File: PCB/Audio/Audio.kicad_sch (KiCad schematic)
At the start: 30 parts, among them J3 TC2030-USB-NL-DS, J4 TF_PUSH, J5 USB-C-Socket-H, U1 L, U2 ESP32-S3-MINI-1, U2 R, U5 MD8942

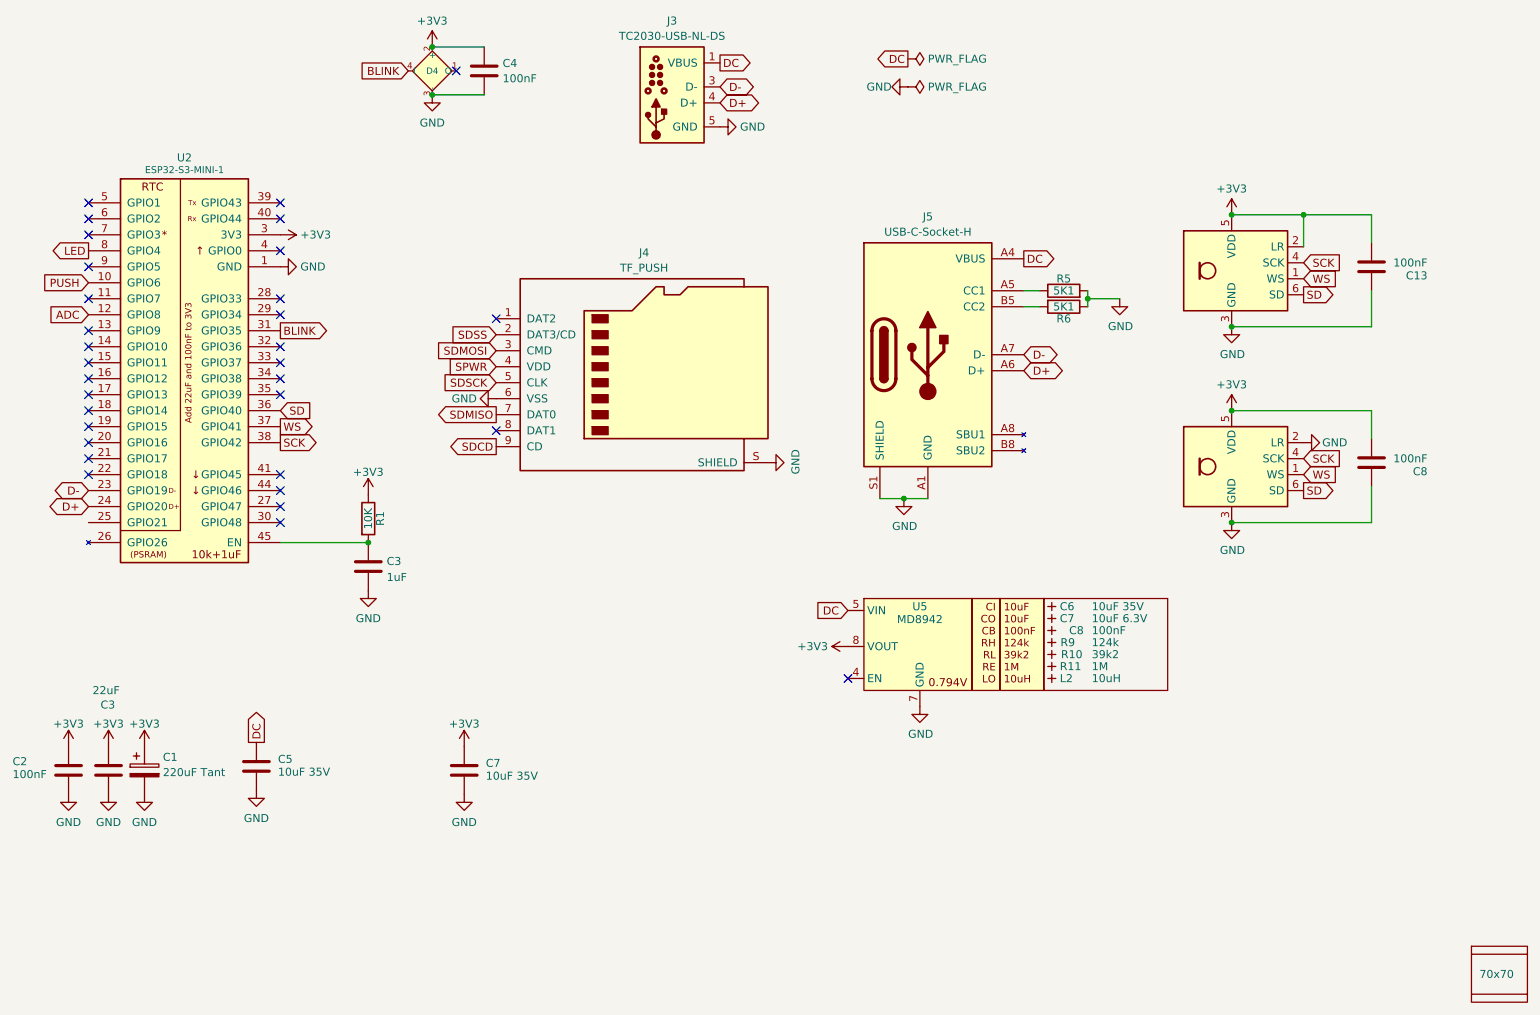
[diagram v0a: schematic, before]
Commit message: Rework concept
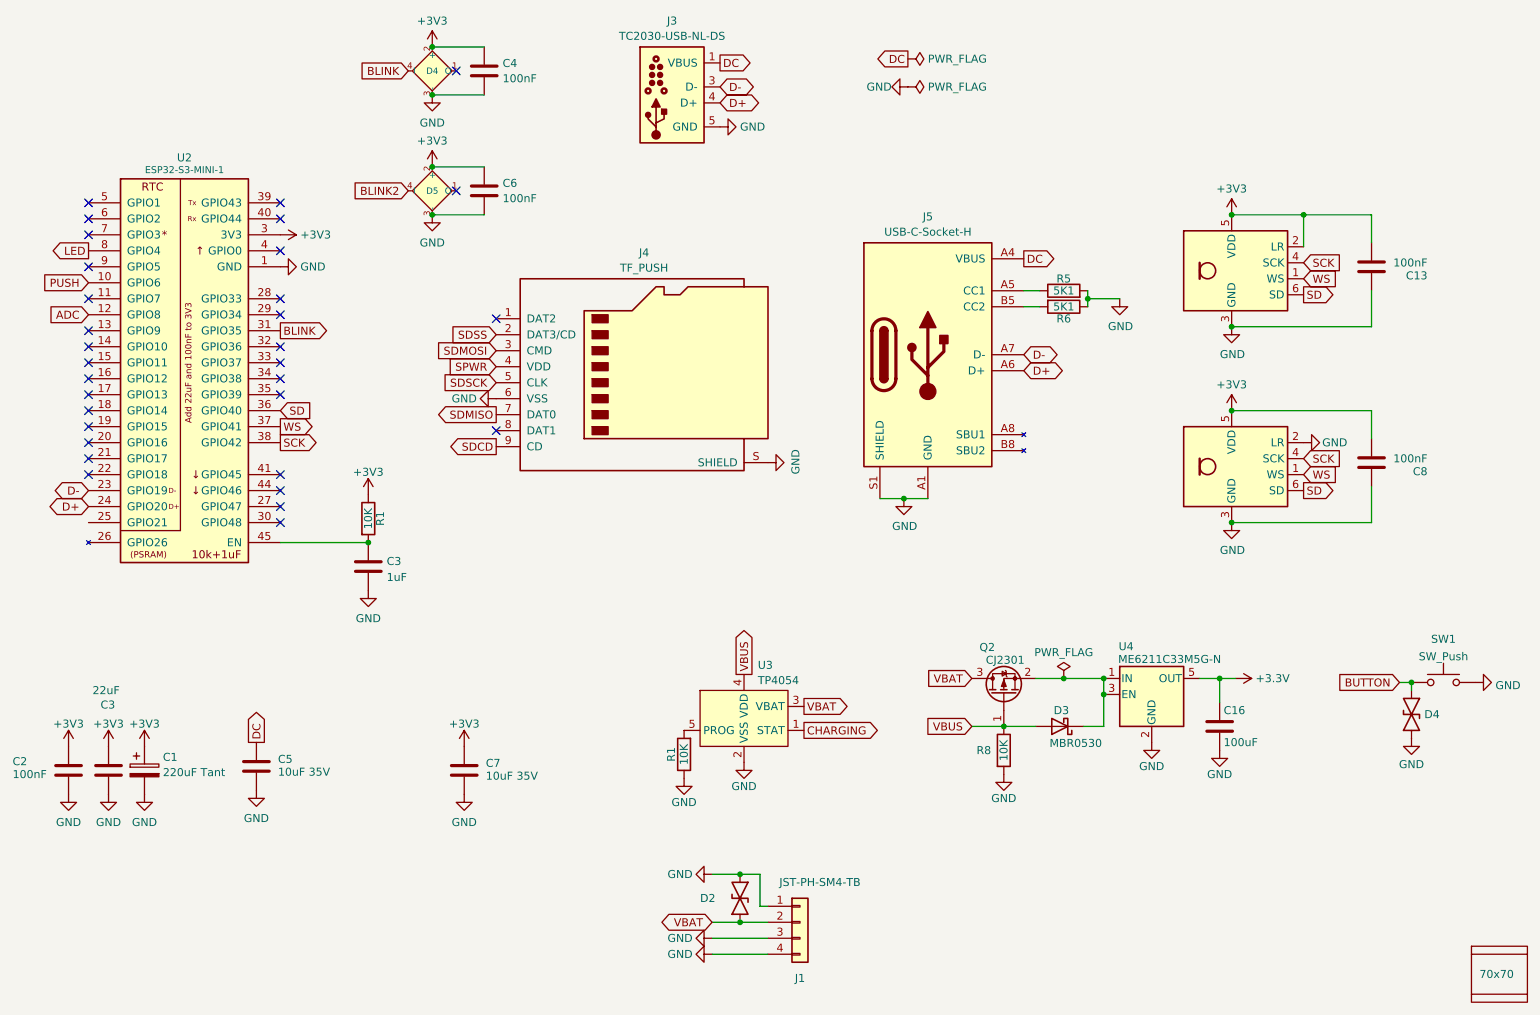
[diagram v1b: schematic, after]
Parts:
- removed C6: 10uF 35V, RevK:C_0603_, symbol RevK:Hidden
- removed C7: 10uF 6.3V, RevK:C_0603_, symbol RevK:Hidden
- removed C8: 100nF, RevK:C_0603_, symbol RevK:Hidden
- removed L2: 10uH, RevK:L_4x4_, symbol RevK:Hidden
- removed R10: 39k2, RevK:R_0402_, symbol RevK:Hidden
- removed R11: 1M, RevK:R_0402_, symbol RevK:Hidden
- removed R9: 124k, RevK:R_0402_, symbol RevK:Hidden
- removed U5: MD8942, RevK:SOT-23-6-MD8942, symbol RevK:MD89420-RegBlock
- added C16: 100uF, RevK:C_0805, symbol Device:C
- added C6: 100nF, RevK:C_0402, symbol Device:C
- added D2, D4: ~, RevK:DFN1006-2L, symbol RevK:ES05D1MC10
- added D3: MBR0530, RevK:D_SOD-123, symbol Device:D_Schottky
- added D5: XL-1010RGBC-WS2812B, RevK:SMD1010, symbol RevK:WS2812B-1mm
- added J1: JST-PH-SM4-TB, RevK:JST_PH_S2B-PH-SM4-TB_1x02-1MP_P2.00mm_Horizontal, symbol Connector_Generic:Conn_01x04
- added Q2: CJ2301, RevK:SOT-23, symbol Transistor_FET:BSS83P
- added R1, R8: 10K, RevK:R_0402, symbol Device:R
- added SW1: SW_Push, RevK:TS-1092S-B3D2-G, symbol Switch:SW_Push
- added U3: TP4054, RevK:SOT-23-5, symbol RevK:TP4054
- added U4: ME6211C33M5G-N, RevK:SOT-23-5, symbol Regulator_Linear:TLV70033_SOT23-5
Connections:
- net +3V3: now also C6.1, D5.2 (+)
- net GND: now also C16.2, C6.2, D2.1, D4.2, D5.3 (-), J1.1 (Pin_1), J1.3 (Pin_3), J1.4 (Pin_4), R1.1, R8.2, SW1.1, U3.2 (VSS), U4.2 (GND)
- new net: D3.1 (K), Q2.2 (S), U4.1 (IN), U4.3 (EN)
- new net: R1.2, U3.5 (PROG)
- new net +3.3V: C16.1, U4.5 (OUT)
- new net BLINK2: D5.4 (I)
- new net BUTTON: D4.1, SW1.2
- new net CHARGING: U3.1 (STAT)
- new net VBAT: D2.2, J1.2 (Pin_2), Q2.3 (D), U3.3 (VBAT)
- new net VBUS: D3.2 (A), Q2.1 (G), R8.1, U3.4 (VDD)
